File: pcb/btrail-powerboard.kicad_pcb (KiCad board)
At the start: 2 copper layers, 44.5 x 52.8 mm, 13 parts, among them J1 RJ45_Shielded, Q1 IRLZ34N, Q2 IRLZ34N

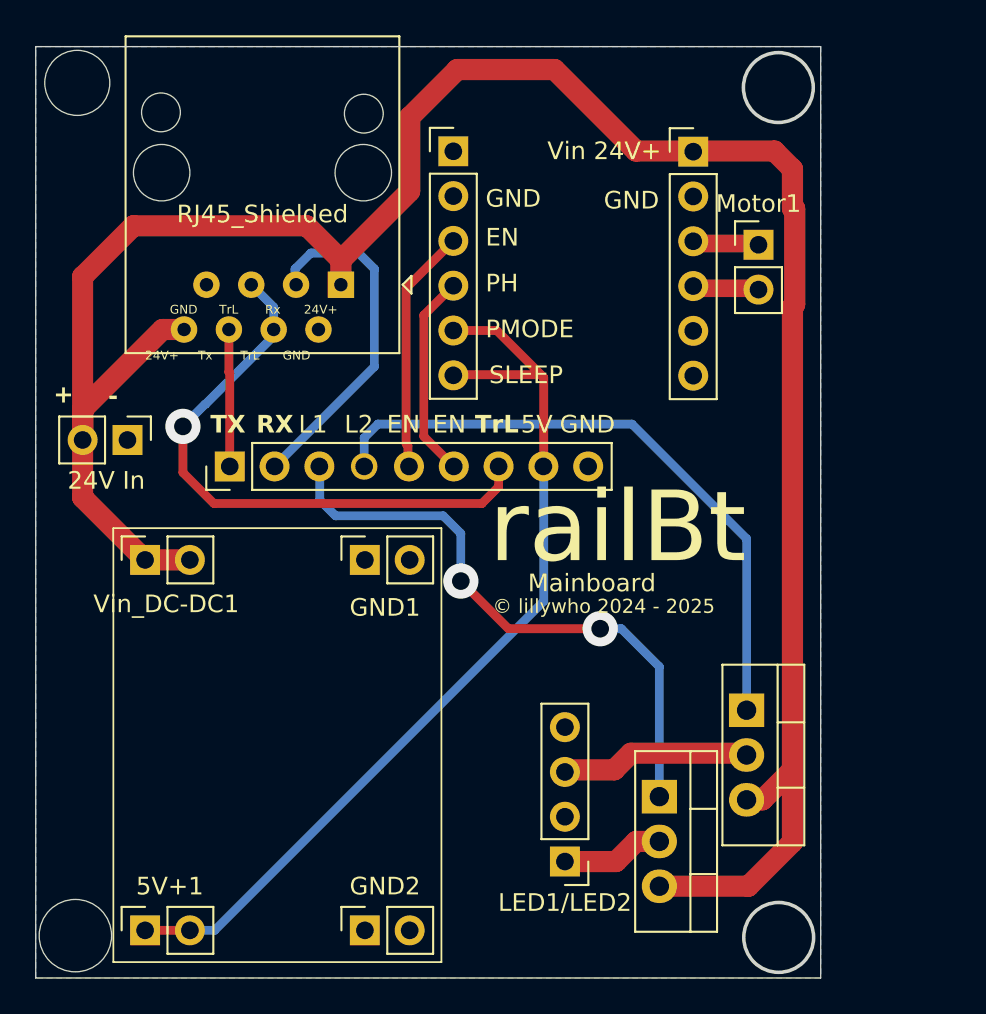
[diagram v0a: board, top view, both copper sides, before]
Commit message: Sync for coop purposes
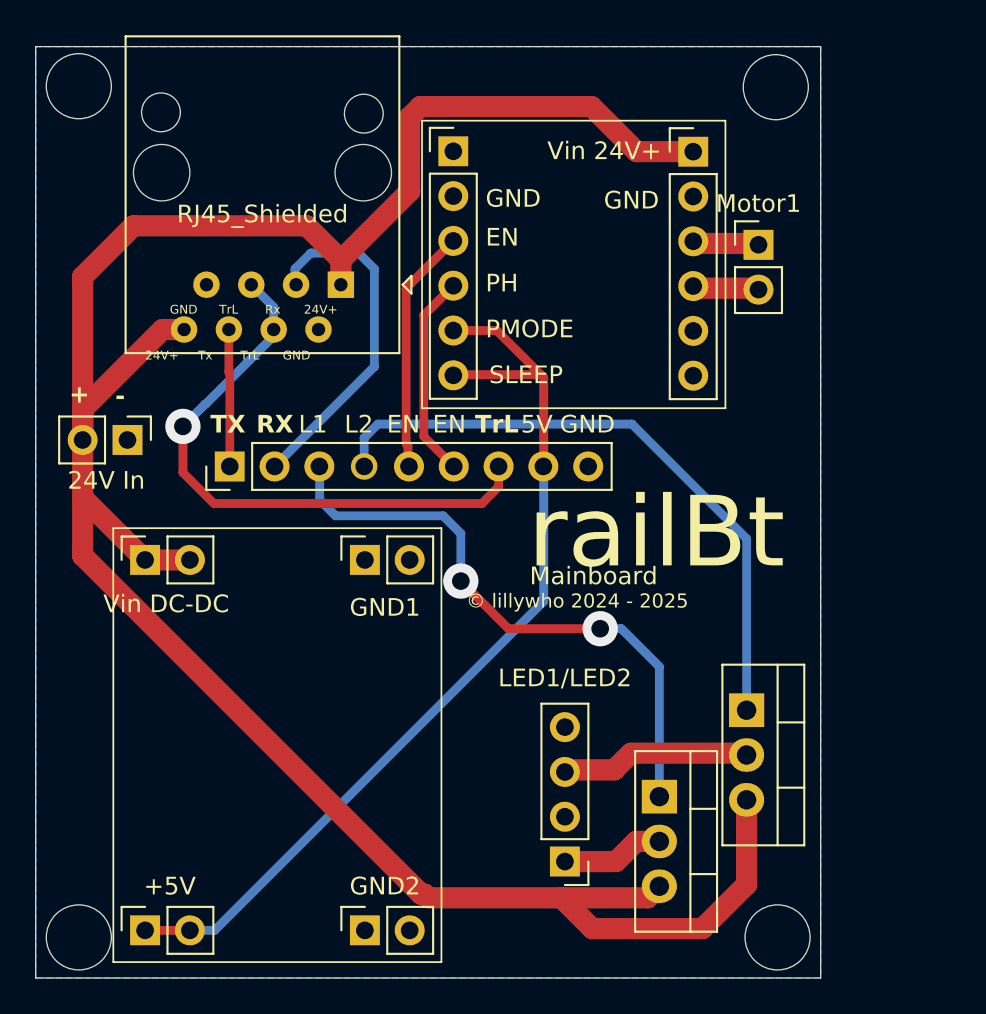
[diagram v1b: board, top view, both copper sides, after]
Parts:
- Vin DC-DC: renamed from Vin_DC-DC1
- renumbered 5V+1 to +5V
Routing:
- net +24V: track 132.6 -> 135.9 mm
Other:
- outline, holes or cut-outs redrawn
